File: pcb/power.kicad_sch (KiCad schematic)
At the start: 29 parts, among them J13 SM04B-SRSS-TB, J2 USB_C_USB2.0_16P, U2 LM66200DRLR, U3 USBLC6-2P6, U6 LM66200DRLR, U7 AZ1084-3.3

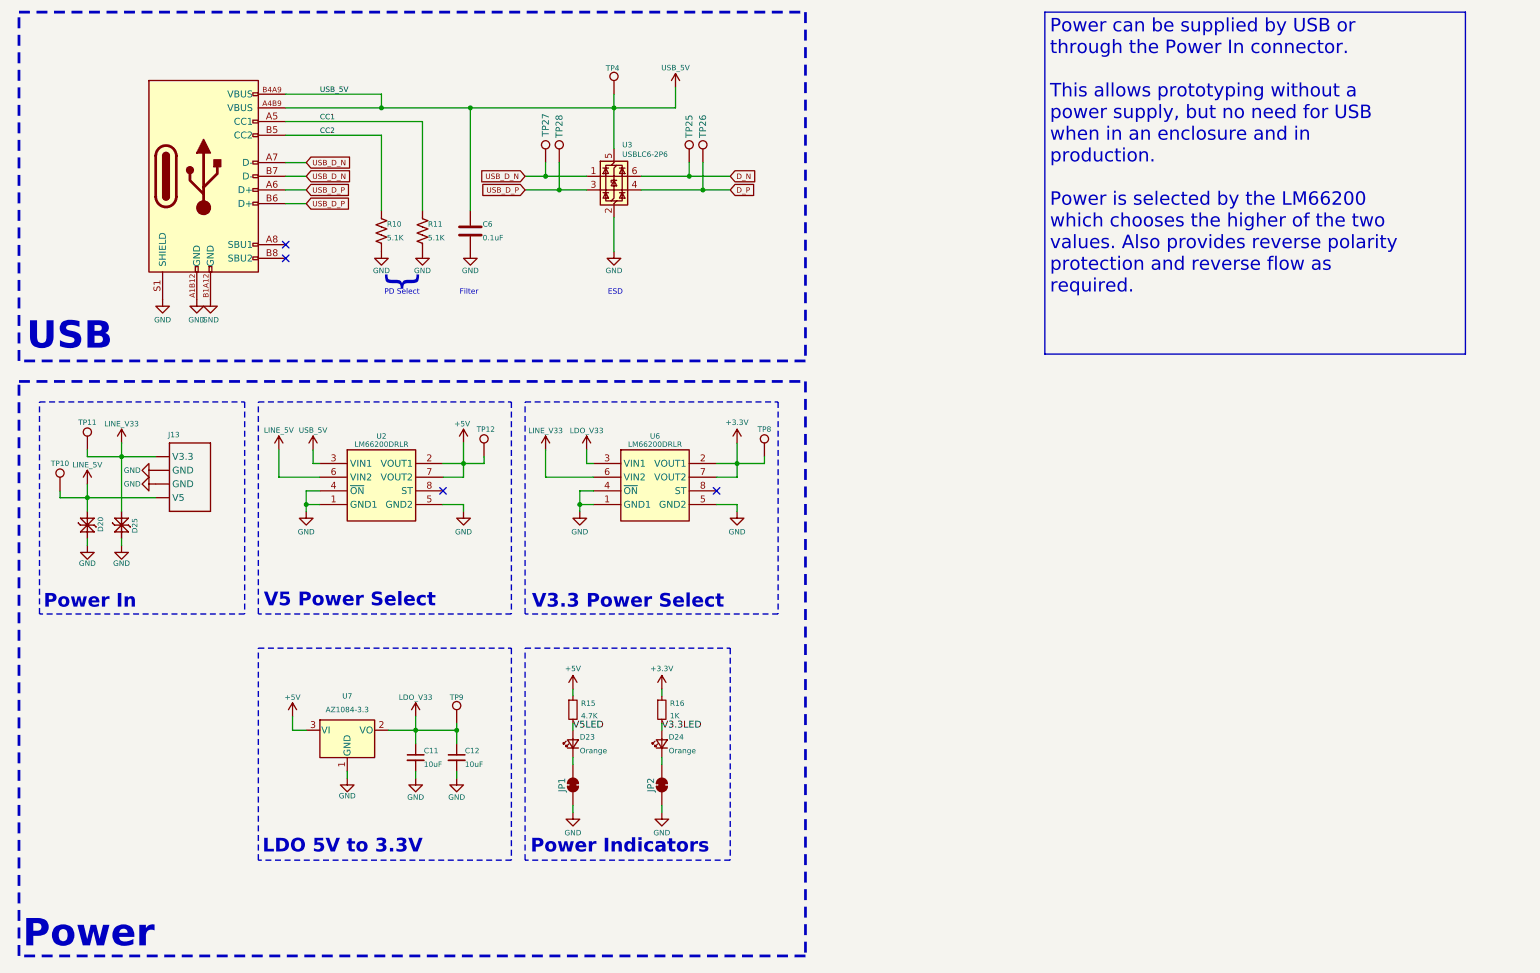
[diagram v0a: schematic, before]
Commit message: Clean up and consistency
Moved buzzer to MCU
Fixed model directory
Set font size
Set outline size
Upscaled Roxy ❤️
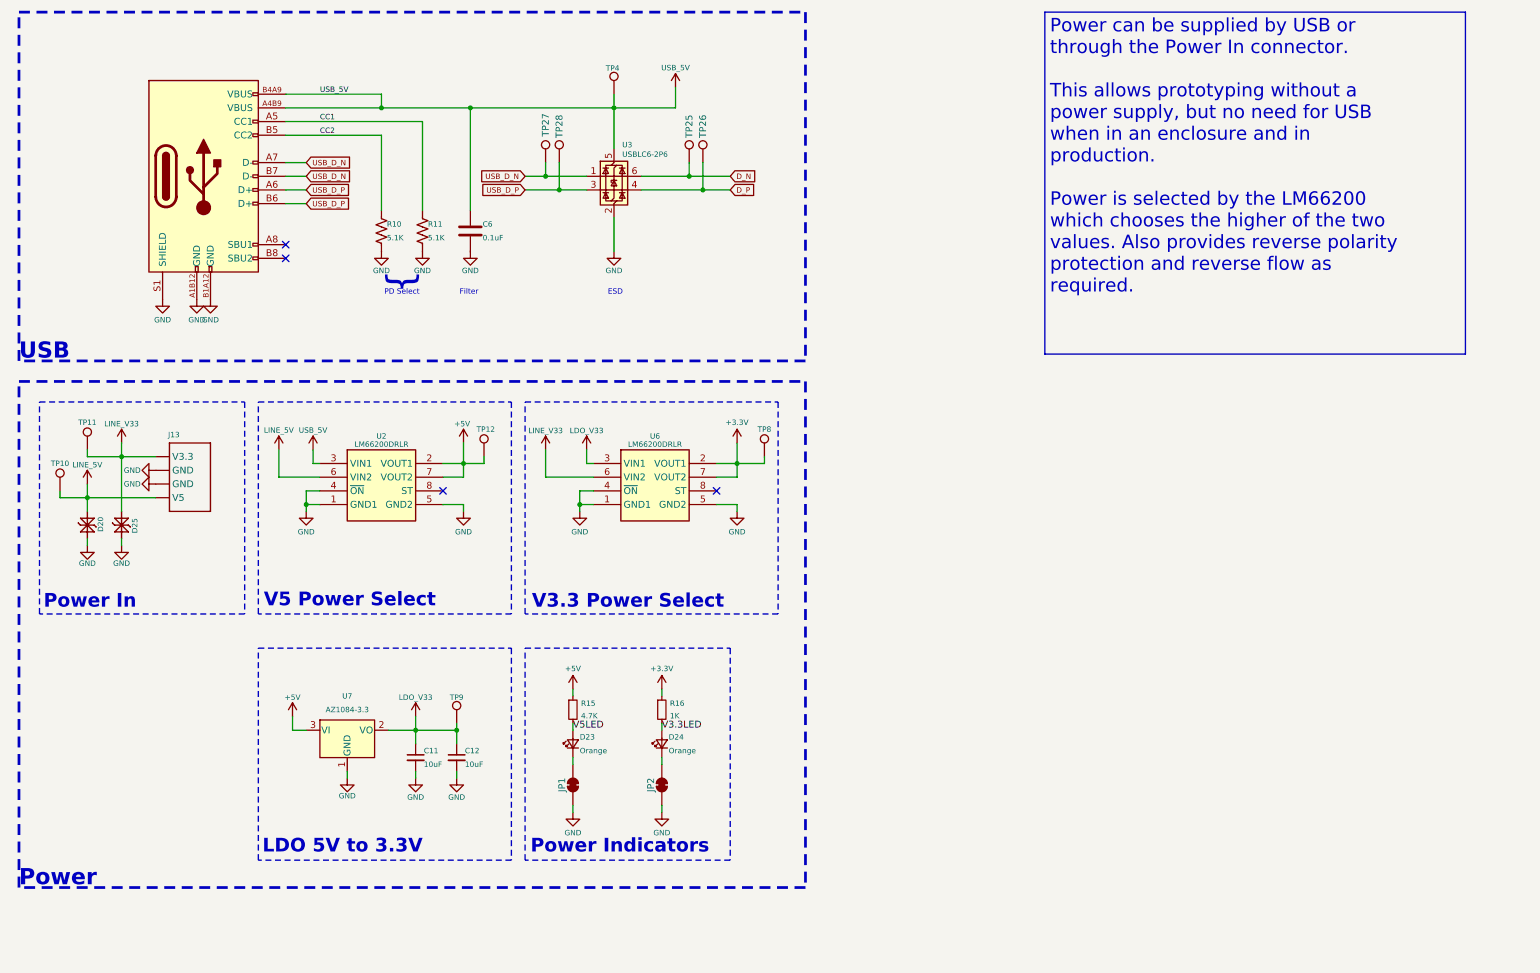
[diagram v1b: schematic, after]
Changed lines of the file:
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@@
 	(rectangle
 		(start 15.24 83.82)
-		(end 161.29 190.5)
+		(end 161.29 177.8)
 		(stroke
 			(width 0.508)
@@
 	(text "USB"
 		(exclude_from_sim yes)
-		(at 24.638 75.438 0)
+		(at 15.24 80.01 0)
 		(effects
 			(font
 				(face "KiCad Font")
-				(size 5.08 5.08)
+				(size 3 3)
 				(thickness 1.016)
 				(bold yes)
-				(color 255 153 0 1)
-			)
+				(color 0 0 194 1)
+			)
+			(justify left bottom)
 		)
 	)
@@
 	(text "Power"
 		(exclude_from_sim yes)
-		(at 28.194 186.436 0)
+		(at 15.24 177.8 0)
 		(effects
 			(font
 				(face "KiCad Font")
-				(size 5.08 5.08)
+				(size 3 3)
 				(thickness 1.016)
 				(bold yes)
-				(color 255 153 0 1)
-			)
-		)
-	)
+				(color 0 0 194 1)
+			)
+			(justify left bottom)
+		)
+	)
